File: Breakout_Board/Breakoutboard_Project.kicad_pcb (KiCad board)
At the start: 2 copper layers, 11 parts, among them U1 ADXL380-2BCCZ-RL7, U2 STM32F411, U3 ICM-40609-D, U4 MMC5983MA, U5 BMP581

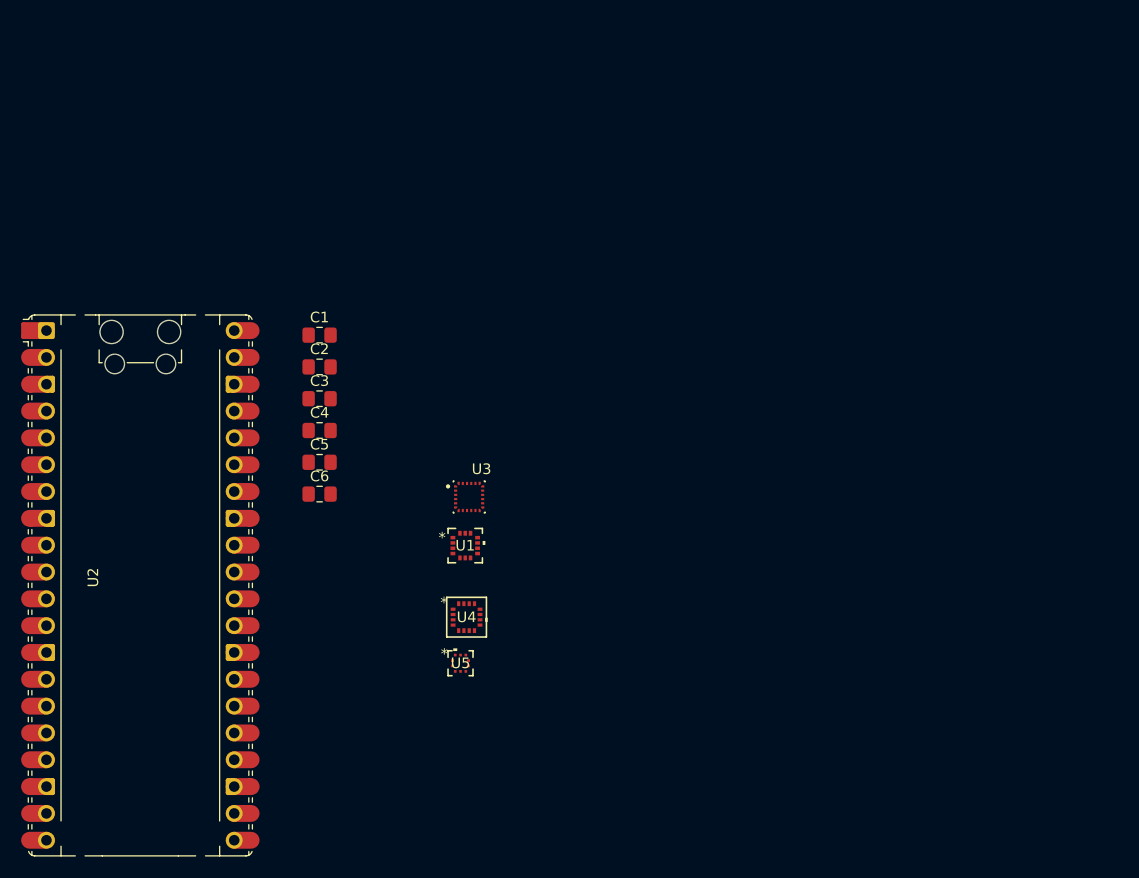
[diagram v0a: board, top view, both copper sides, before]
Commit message: changing around some things
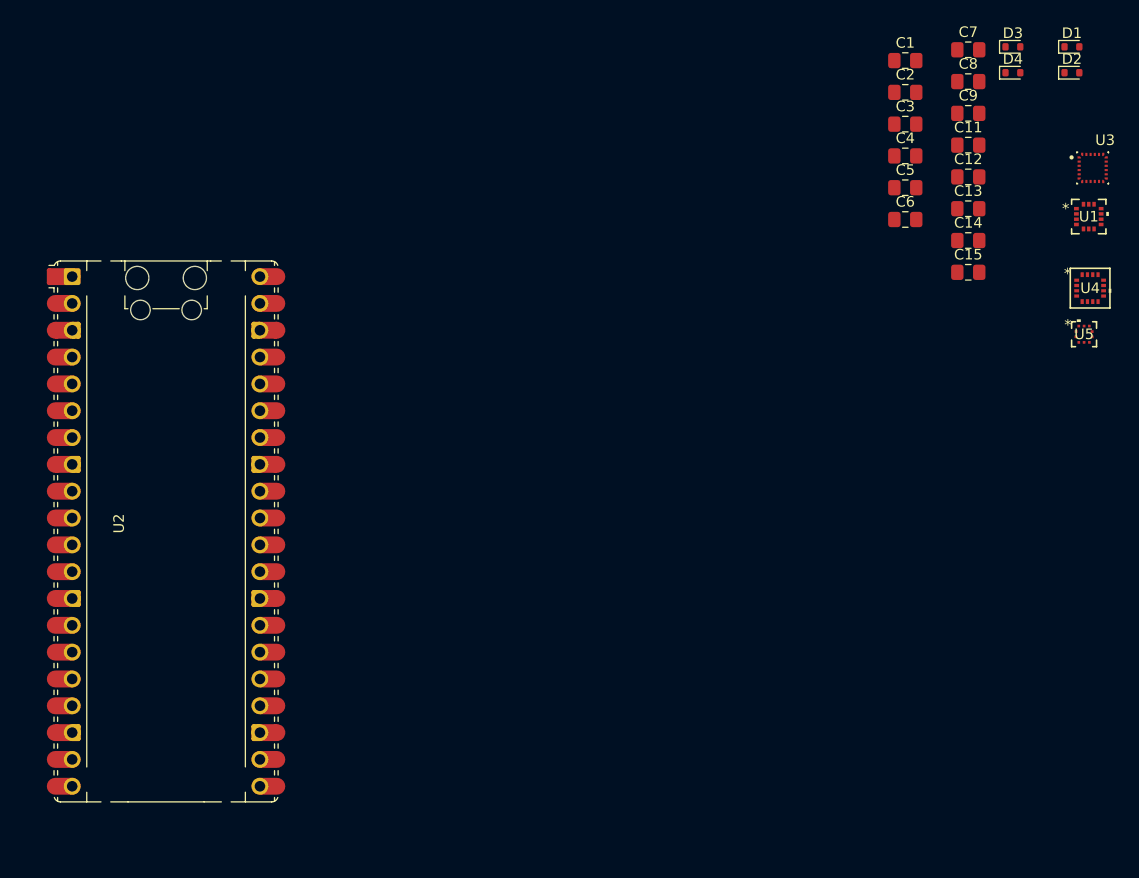
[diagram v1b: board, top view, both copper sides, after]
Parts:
- added C11: .1uf, Capacitor_SMD:C_0805_2012Metric_Pad1.18x1.45mm_HandSolder, F.Cu at (115.0, 23.5)
- added C12: .1uf, Capacitor_SMD:C_0805_2012Metric_Pad1.18x1.45mm_HandSolder, F.Cu at (115.0, 26.5)
- added C13: .1uf, Capacitor_SMD:C_0805_2012Metric_Pad1.18x1.45mm_HandSolder, F.Cu at (115.0, 29.5)
- added C14: 1uf, Capacitor_SMD:C_0805_2012Metric_Pad1.18x1.45mm_HandSolder, F.Cu at (115.0, 32.5)
- added C15: 1uf, Capacitor_SMD:C_0805_2012Metric_Pad1.18x1.45mm_HandSolder, F.Cu at (115.0, 35.5)
- added C7: .1uf, Capacitor_SMD:C_0805_2012Metric_Pad1.18x1.45mm_HandSolder, F.Cu at (115.0, 14.4)
- added C8: 1uf, Capacitor_SMD:C_0805_2012Metric_Pad1.18x1.45mm_HandSolder, F.Cu at (115.0, 17.4)
- added C9: 10uf, Capacitor_SMD:C_0805_2012Metric_Pad1.18x1.45mm_HandSolder, F.Cu at (115.0, 20.4)
- added D1: ESD5Zxx, Diode_SMD:D_SOD-523, F.Cu at (124.8, 14.2)
- added D2: ESD5Zxx, Diode_SMD:D_SOD-523, F.Cu at (124.8, 16.6)
- added D3: ESD5Zxx, Diode_SMD:D_SOD-523, F.Cu at (119.2, 14.2)
- added D4: ESD5Zxx, Diode_SMD:D_SOD-523, F.Cu at (119.2, 16.6)
- moved U1 66.8 mm to (126.4, 30.2)
- moved U3 66.8 mm to (126.7, 25.6)
- moved U4 66.8 mm to (126.5, 37.0)
- moved U5 66.8 mm to (125.9, 41.4)
- moved C1 61.3 mm to (109.0, 15.4)
- moved C5 61.3 mm to (109.0, 27.5)
- moved C2 61.3 mm to (109.0, 18.5)
- moved C3 61.3 mm to (109.0, 21.5)
- moved C4 61.3 mm to (109.0, 24.5)
- moved C6 61.3 mm to (109.0, 30.5)
- moved U2 5.66 mm to (37.9, 59.5)
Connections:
- U1 pad 1: unconnected-(U1-FSYNC-Pad1) -> /Accel & Gyro/FSYNC_ADXL
- U1 pad 10: unconnected-(U1-VS-Pad10) -> +3.3V
- U1 pad 11: unconnected-(U1-VDDIO-Pad11) -> +3.3V
- U1 pad 2: unconnected-(U1-SCLK/SCL-Pad2) -> /SCLK_Accel_gyro
- U1 pad 3: unconnected-(U1-SDI/SDA-Pad3) -> /MOSI_Accel_gyro
- U1 pad 4: unconnected-(U1-SDO/ASEL0-Pad4) -> /MISO_Accel_gyro
- U1 pad 5: unconnected-(U1-*CS/ASEL1-Pad5) -> /CS_ADXL
- U1 pad 6: unconnected-(U1-INT0-Pad6) -> /Accel & Gyro/INT0_ADXL
- U1 pad 7: unconnected-(U1-INT1-Pad7) -> /Accel & Gyro/INT1_ADXL
- U1 pad 8: unconnected-(U1-V1P8-Pad8) -> Net-(U1-V1P8)
- U1 pad 9: unconnected-(U1-GND-Pad9) -> GND
- U2 pad 29: unconnected-(U2-A3-Pad29) -> /CS_ADXL
- U2 pad 30: unconnected-(U2-A4-Pad30) -> /CS_ICM
- U2 pad 31: unconnected-(U2-A5-Pad31) -> /SCLK_Accel_gyro
- U2 pad 32: unconnected-(U2-A6-Pad32) -> /MISO_Accel_gyro
- U2 pad 33: unconnected-(U2-A7-Pad33) -> /MOSI_Accel_gyro
- U3 pad 11: unconnected-(U3-RESV-Pad11) -> GND
- U3 pad 12: unconnected-(U3-INT1/INT-Pad12) -> /Accel & Gyro/INT1_ICM
- U3 pad 13: unconnected-(U3-VDD-Pad13) -> +3.3V
- U3 pad 18: unconnected-(U3-GND-Pad18) -> GND
- U3 pad 19: unconnected-(U3-INT2/FSYNC-Pad19) -> /Accel & Gyro/FSYNC_ICM
- U3 pad 20: unconnected-(U3-RESV__1-Pad20) -> GND
- U3 pad 22: unconnected-(U3-~{CS}-Pad22) -> /CS_ICM
- U3 pad 23: unconnected-(U3-SCL/SCLK-Pad23) -> /SCLK_Accel_gyro
- U3 pad 24: unconnected-(U3-SDA/SDI/SDIO-Pad24) -> /MOSI_Accel_gyro
- U3 pad 8: unconnected-(U3-VDDIO-Pad8) -> +3.3V
- U3 pad 9: unconnected-(U3-AD0/SDO-Pad9) -> /MISO_Accel_gyro
